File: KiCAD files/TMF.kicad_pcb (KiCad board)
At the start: 2 copper layers, 100 x 99.5 mm, 90 parts, among them J1 Conn_01x04_Pin, J2 Conn_01x04_Pin

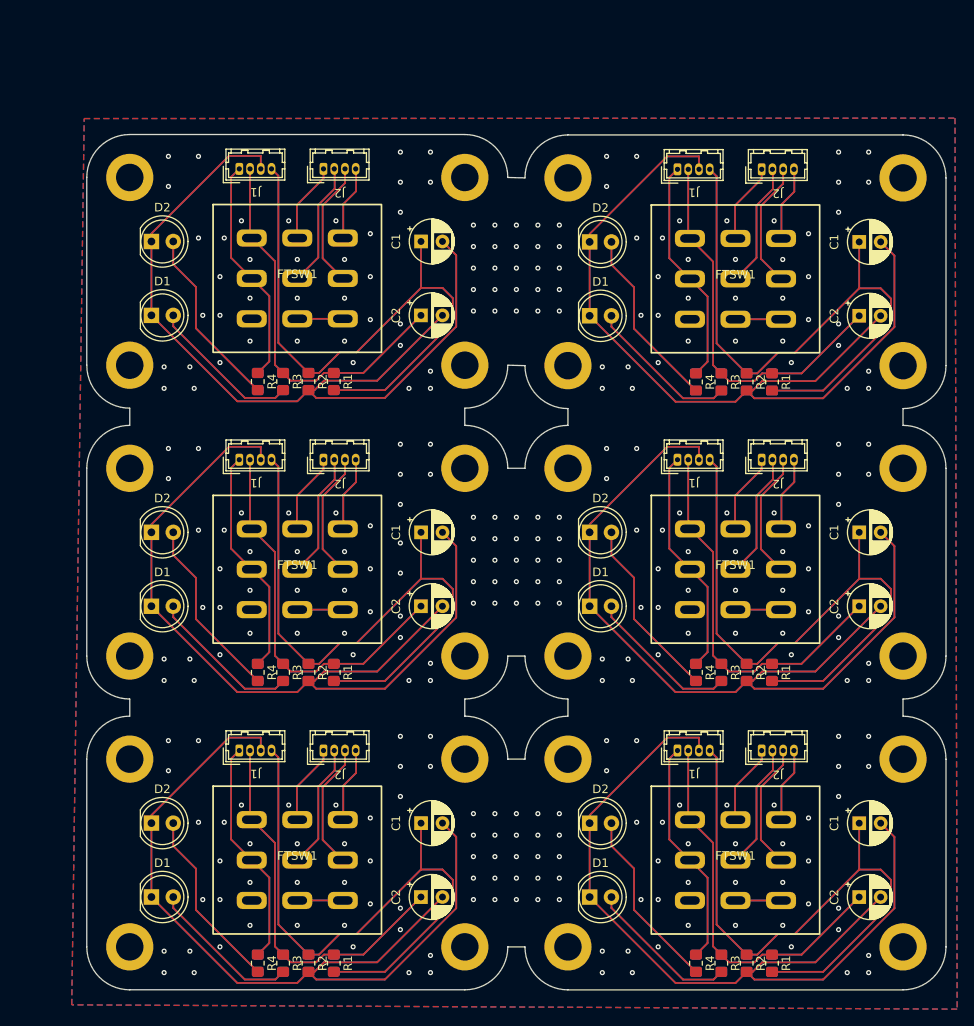
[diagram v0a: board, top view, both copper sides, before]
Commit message: Redone PCB
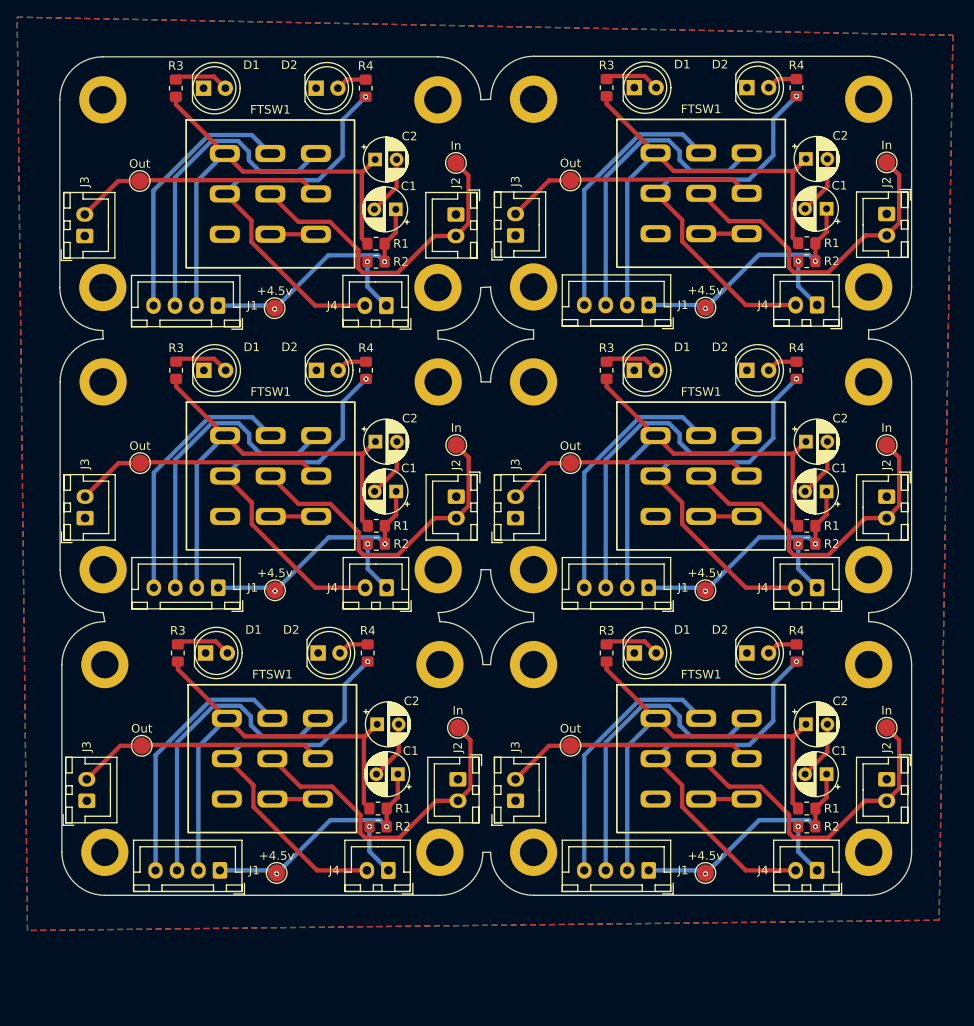
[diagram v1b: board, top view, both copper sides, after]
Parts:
- removed the ? at (167.0, 126.0)
- removed the ? at (167.0, 92.2)
- removed the ? at (116.0, 58.3)
- removed the ? at (167.0, 104.2)
- removed the ? at (116.0, 70.3)
- removed the ? at (116.0, 92.2)
- removed the ? at (116.0, 36.5)
- removed the ? at (167.0, 58.4)
- removed the ? at (167.0, 70.3)
- removed the ? at (167.0, 36.5)
- removed the C1 at (149.9, 43.9)
- removed the C1 at (149.9, 111.6)
- removed the C1 at (149.9, 77.8)
- removed the C1 at (200.9, 111.6)
- removed the C1 at (200.9, 44.0)
- removed the C1 at (200.9, 77.8)
- removed the C2 at (200.9, 86.4)
- removed the C2 at (149.9, 120.2)
- removed the C2 at (149.9, 52.5)
- removed the C2 at (149.9, 86.4)
- removed the C2 at (200.9, 120.2)
- removed the C2 at (200.9, 52.6)
- removed the D1 at (118.5, 86.4)
- removed the D1 at (118.5, 52.5)
- removed the D1 at (118.5, 120.2)
- removed the D1 at (169.5, 120.2)
- removed the D1 at (169.5, 86.4)
- removed the D1 at (169.5, 52.6)
- removed the D2 at (118.5, 77.8)
- removed the D2 at (118.5, 43.9)
- removed the D2 at (169.5, 111.6)
- removed the D2 at (118.5, 111.6)
- removed the D2 at (169.5, 77.8)
- removed the D2 at (169.5, 44.0)
- removed the FTSW1 at (135.5, 48.2)
- removed the FTSW1 at (186.5, 115.9)
- removed the FTSW1 at (135.5, 115.9)
- removed the FTSW1 at (186.5, 48.3)
- removed the FTSW1 at (186.5, 82.1)
- removed the FTSW1 at (135.5, 82.1)
- removed the J1 at (179.8, 35.5)
- removed the J1 at (128.8, 35.5)
- removed the J1 at (179.8, 103.2)
- removed the J1 at (128.8, 69.3)
- removed the J1 at (179.8, 69.3)
- removed the J1 at (128.8, 103.2)
- removed the J2 at (138.6, 35.5)
- removed the J2 at (189.6, 35.5)
- removed the J2 at (138.6, 69.3)
- removed the J2 at (138.6, 103.2)
- removed the J2 at (189.6, 103.2)
- removed the J2 at (189.6, 69.3)
- removed the R1 at (190.8, 60.3)
- removed the R1 at (190.8, 94.1)
- removed the R1 at (139.8, 127.9)
- removed the R1 at (139.8, 94.1)
- removed the R1 at (139.8, 60.2)
- removed the R1 at (190.8, 127.9)
- removed the R2 at (136.8, 94.1)
- removed the R2 at (187.8, 94.1)
- removed the R2 at (136.8, 60.2)
- removed the R2 at (187.8, 127.9)
- removed the R2 at (136.8, 127.9)
- removed the R2 at (187.8, 60.3)
- removed the R3 at (184.8, 94.1)
- removed the R3 at (133.8, 94.1)
- removed the R3 at (184.8, 127.9)
- removed the R3 at (133.8, 127.9)
- removed the R3 at (133.8, 60.2)
- removed the R3 at (184.8, 60.3)
- removed the R4 at (130.9, 60.2)
- removed the R4 at (181.9, 60.3)
- removed the R4 at (181.9, 127.9)
- removed the R4 at (130.9, 94.1)
- removed the R4 at (130.9, 127.9)
- removed the R4 at (181.9, 94.1)
- removed the REF** at (206.0, 70.3)
- removed the REF** at (155.0, 92.2)
- removed the REF** at (155.0, 70.3)
- removed the REF** at (206.0, 104.2)
- removed the REF** at (155.0, 58.3)
- removed the REF** at (206.0, 92.2)
- removed the REF** at (206.0, 58.4)
- removed the REF** at (206.0, 36.5)
- removed the REF** at (155.0, 36.5)
- removed the REF** at (206.0, 126.0)
- added +4.5v: TestPoint_Pad_D2.0mm, TestPoint:TestPoint_Pad_D2.0mm, F.Cu at (183.0, 117.4)
- added +4.5v: TestPoint_Pad_D2.0mm, TestPoint:TestPoint_Pad_D2.0mm, F.Cu at (132.9, 51.7)
- added +4.5v: TestPoint_Pad_D2.0mm, TestPoint:TestPoint_Pad_D2.0mm, F.Cu at (183.0, 51.6)
- added +4.5v: TestPoint_Pad_D2.0mm, TestPoint:TestPoint_Pad_D2.0mm, F.Cu at (183.0, 84.5)
- added +4.5v: TestPoint_Pad_D2.0mm, TestPoint:TestPoint_Pad_D2.0mm, F.Cu at (132.9, 84.5)
- added +4.5v: TestPoint_Pad_D2.0mm, TestPoint:TestPoint_Pad_D2.0mm, F.Cu at (133.1, 117.4)
- added ?: , , F.Cu at (112.9, 82.1)
- added ?: , , F.Cu at (112.9, 27.4)
- added ?: , , F.Cu at (112.9, 49.3)
- added ?: , , F.Cu at (163.0, 49.2)
- added ?: , , F.Cu at (163.0, 27.3)
- added ?: , , F.Cu at (163.0, 93.1)
- added ?: , , F.Cu at (163.0, 115.0)
- added ?: , , F.Cu at (112.9, 60.2)
- added ?: , , F.Cu at (163.0, 60.2)
- added ?: , , F.Cu at (163.0, 82.1)
- added C1: 10µF, Capacitor_THT:CP_Radial_D5.0mm_P2.50mm, F.Cu at (197.1, 40.1)
- added C1: 10µF, Capacitor_THT:CP_Radial_D5.0mm_P2.50mm, F.Cu at (147.0, 73.0)
- added C1: 10µF, Capacitor_THT:CP_Radial_D5.0mm_P2.50mm, F.Cu at (147.0, 40.2)
- added C1: 10µF, Capacitor_THT:CP_Radial_D5.0mm_P2.50mm, F.Cu at (147.2, 105.9)
- added C1: 10µF, Capacitor_THT:CP_Radial_D5.0mm_P2.50mm, F.Cu at (197.1, 105.9)
- added C1: 10µF, Capacitor_THT:CP_Radial_D5.0mm_P2.50mm, F.Cu at (197.1, 73.0)
- added C2: 100µF, Capacitor_THT:CP_Radial_D5.0mm_P2.50mm, F.Cu at (194.7, 34.3)
- added C2: 100µF, Capacitor_THT:CP_Radial_D5.0mm_P2.50mm, F.Cu at (194.7, 67.2)
- added C2: 100µF, Capacitor_THT:CP_Radial_D5.0mm_P2.50mm, F.Cu at (144.8, 100.1)
- added C2: 100µF, Capacitor_THT:CP_Radial_D5.0mm_P2.50mm, F.Cu at (194.7, 100.1)
- added C2: 100µF, Capacitor_THT:CP_Radial_D5.0mm_P2.50mm, F.Cu at (144.6, 34.4)
- added C2: 100µF, Capacitor_THT:CP_Radial_D5.0mm_P2.50mm, F.Cu at (144.6, 67.2)
- added D1: EFFECT, LED_THT:LED_D5.0mm_Clear, F.Cu at (124.6, 58.9)
- added D1: EFFECT, LED_THT:LED_D5.0mm_Clear, F.Cu at (174.7, 58.9)
- added D1: EFFECT, LED_THT:LED_D5.0mm_Clear, F.Cu at (124.8, 91.8)
- added D1: EFFECT, LED_THT:LED_D5.0mm_Clear, F.Cu at (174.7, 91.8)
- added D1: EFFECT, LED_THT:LED_D5.0mm_Clear, F.Cu at (124.6, 26.1)
- added D1: EFFECT, LED_THT:LED_D5.0mm_Clear, F.Cu at (174.7, 26.0)
- added D2: POW, LED_THT:LED_D5.0mm_Clear, F.Cu at (137.9, 91.8)
- added D2: POW, LED_THT:LED_D5.0mm_Clear, F.Cu at (137.7, 58.9)
- added D2: POW, LED_THT:LED_D5.0mm_Clear, F.Cu at (187.8, 58.9)
- added D2: POW, LED_THT:LED_D5.0mm_Clear, F.Cu at (187.8, 91.8)
- added D2: POW, LED_THT:LED_D5.0mm_Clear, F.Cu at (187.8, 26.0)
- added D2: POW, LED_THT:LED_D5.0mm_Clear, F.Cu at (137.7, 26.1)
- added FTSW1: ~, Footswitch:3PDT Footswitch, F.Cu at (132.6, 104.1)
- added FTSW1: ~, Footswitch:3PDT Footswitch, F.Cu at (182.5, 38.3)
- added FTSW1: ~, Footswitch:3PDT Footswitch, F.Cu at (182.5, 104.1)
- added FTSW1: ~, Footswitch:3PDT Footswitch, F.Cu at (132.4, 38.4)
- added FTSW1: ~, Footswitch:3PDT Footswitch, F.Cu at (182.5, 71.2)
- added FTSW1: ~, Footswitch:3PDT Footswitch, F.Cu at (132.4, 71.2)
- added In: TestPoint_Pad_D2.0mm, TestPoint:TestPoint_Pad_D2.0mm, F.Cu at (204.1, 34.7)
- added In: TestPoint_Pad_D2.0mm, TestPoint:TestPoint_Pad_D2.0mm, F.Cu at (154.0, 67.6)
- added In: TestPoint_Pad_D2.0mm, TestPoint:TestPoint_Pad_D2.0mm, F.Cu at (154.2, 100.5)
- added In: TestPoint_Pad_D2.0mm, TestPoint:TestPoint_Pad_D2.0mm, F.Cu at (204.1, 100.5)
- added In: TestPoint_Pad_D2.0mm, TestPoint:TestPoint_Pad_D2.0mm, F.Cu at (204.1, 67.6)
- added In: TestPoint_Pad_D2.0mm, TestPoint:TestPoint_Pad_D2.0mm, F.Cu at (154.0, 34.8)
- added J1: DST-2, Connector_JST:JST_XH_B4B-XH-A_1x04_P2.50mm_Vertical, F.Cu at (126.3, 51.4)
- added J1: DST-2, Connector_JST:JST_XH_B4B-XH-A_1x04_P2.50mm_Vertical, F.Cu at (176.4, 117.1)
- added J1: DST-2, Connector_JST:JST_XH_B4B-XH-A_1x04_P2.50mm_Vertical, F.Cu at (126.5, 117.1)
- added J1: DST-2, Connector_JST:JST_XH_B4B-XH-A_1x04_P2.50mm_Vertical, F.Cu at (176.4, 51.3)
- added J1: DST-2, Connector_JST:JST_XH_B4B-XH-A_1x04_P2.50mm_Vertical, F.Cu at (126.3, 84.2)
- added J1: DST-2, Connector_JST:JST_XH_B4B-XH-A_1x04_P2.50mm_Vertical, F.Cu at (176.4, 84.2)
- added J2: TMC-1, Connector_JST:JST_XH_B2B-XH-A_1x02_P2.50mm_Vertical, F.Cu at (154.2, 106.5)
- added J2: TMC-1, Connector_JST:JST_XH_B2B-XH-A_1x02_P2.50mm_Vertical, F.Cu at (204.1, 106.5)
- added J2: TMC-1, Connector_JST:JST_XH_B2B-XH-A_1x02_P2.50mm_Vertical, F.Cu at (204.1, 40.7)
- added J2: TMC-1, Connector_JST:JST_XH_B2B-XH-A_1x02_P2.50mm_Vertical, F.Cu at (154.0, 73.6)
- added J2: TMC-1, Connector_JST:JST_XH_B2B-XH-A_1x02_P2.50mm_Vertical, F.Cu at (204.1, 73.6)
- added J2: TMC-1, Connector_JST:JST_XH_B2B-XH-A_1x02_P2.50mm_Vertical, F.Cu at (154.0, 40.8)
- added J3: TMC-1, Connector_JST:JST_XH_B2B-XH-A_1x02_P2.50mm_Vertical, F.Cu at (160.9, 43.2)
- added J3: TMC-1, Connector_JST:JST_XH_B2B-XH-A_1x02_P2.50mm_Vertical, F.Cu at (160.9, 76.1)
- added J3: TMC-1, Connector_JST:JST_XH_B2B-XH-A_1x02_P2.50mm_Vertical, F.Cu at (160.9, 109.0)
- added J3: TMC-1, Connector_JST:JST_XH_B2B-XH-A_1x02_P2.50mm_Vertical, F.Cu at (110.8, 43.3)
- added J3: TMC-1, Connector_JST:JST_XH_B2B-XH-A_1x02_P2.50mm_Vertical, F.Cu at (111.0, 109.0)
- added J3: TMC-1, Connector_JST:JST_XH_B2B-XH-A_1x02_P2.50mm_Vertical, F.Cu at (110.8, 76.1)
- added J4: DST-2, Connector_JST:JST_XH_B2B-XH-A_1x02_P2.50mm_Vertical, F.Cu at (145.9, 51.4)
- added J4: DST-2, Connector_JST:JST_XH_B2B-XH-A_1x02_P2.50mm_Vertical, F.Cu at (196.0, 84.2)
- added J4: DST-2, Connector_JST:JST_XH_B2B-XH-A_1x02_P2.50mm_Vertical, F.Cu at (196.0, 117.1)
- added J4: DST-2, Connector_JST:JST_XH_B2B-XH-A_1x02_P2.50mm_Vertical, F.Cu at (145.9, 84.2)
- added J4: DST-2, Connector_JST:JST_XH_B2B-XH-A_1x02_P2.50mm_Vertical, F.Cu at (196.0, 51.3)
- added J4: DST-2, Connector_JST:JST_XH_B2B-XH-A_1x02_P2.50mm_Vertical, F.Cu at (146.1, 117.1)
- added Out: TestPoint_Pad_D2.0mm, TestPoint:TestPoint_Pad_D2.0mm, F.Cu at (167.3, 36.8)
- added Out: TestPoint_Pad_D2.0mm, TestPoint:TestPoint_Pad_D2.0mm, F.Cu at (117.4, 102.6)
- added Out: TestPoint_Pad_D2.0mm, TestPoint:TestPoint_Pad_D2.0mm, F.Cu at (117.2, 36.9)
- added Out: TestPoint_Pad_D2.0mm, TestPoint:TestPoint_Pad_D2.0mm, F.Cu at (117.2, 69.7)
- added Out: TestPoint_Pad_D2.0mm, TestPoint:TestPoint_Pad_D2.0mm, F.Cu at (167.3, 69.7)
- added Out: TestPoint_Pad_D2.0mm, TestPoint:TestPoint_Pad_D2.0mm, F.Cu at (167.3, 102.6)
- added R1: 10kΩ, Resistor_SMD:R_0805_2012Metric_Pad1.20x1.40mm_HandSolder, F.Cu at (194.8, 77.0)
- added R1: 10kΩ, Resistor_SMD:R_0805_2012Metric_Pad1.20x1.40mm_HandSolder, F.Cu at (144.9, 109.9)
- added R1: 10kΩ, Resistor_SMD:R_0805_2012Metric_Pad1.20x1.40mm_HandSolder, F.Cu at (194.8, 109.9)
- added R1: 10kΩ, Resistor_SMD:R_0805_2012Metric_Pad1.20x1.40mm_HandSolder, F.Cu at (144.7, 44.2)
- added R1: 10kΩ, Resistor_SMD:R_0805_2012Metric_Pad1.20x1.40mm_HandSolder, F.Cu at (144.7, 77.0)
- added R1: 10kΩ, Resistor_SMD:R_0805_2012Metric_Pad1.20x1.40mm_HandSolder, F.Cu at (194.8, 44.1)
- added R2: 10kΩ, Resistor_SMD:R_0805_2012Metric_Pad1.20x1.40mm_HandSolder, F.Cu at (194.8, 46.2)
- added R2: 10kΩ, Resistor_SMD:R_0805_2012Metric_Pad1.20x1.40mm_HandSolder, F.Cu at (144.7, 46.3)
- added R2: 10kΩ, Resistor_SMD:R_0805_2012Metric_Pad1.20x1.40mm_HandSolder, F.Cu at (194.8, 112.0)
- added R2: 10kΩ, Resistor_SMD:R_0805_2012Metric_Pad1.20x1.40mm_HandSolder, F.Cu at (194.8, 79.1)
- added R2: 10kΩ, Resistor_SMD:R_0805_2012Metric_Pad1.20x1.40mm_HandSolder, F.Cu at (144.7, 79.1)
- added R2: 10kΩ, Resistor_SMD:R_0805_2012Metric_Pad1.20x1.40mm_HandSolder, F.Cu at (144.9, 112.0)
- added R3: 1kΩ, Resistor_SMD:R_0805_2012Metric_Pad1.20x1.40mm_HandSolder, F.Cu at (171.5, 26.0)
- added R3: 1kΩ, Resistor_SMD:R_0805_2012Metric_Pad1.20x1.40mm_HandSolder, F.Cu at (171.5, 58.9)
- added R3: 1kΩ, Resistor_SMD:R_0805_2012Metric_Pad1.20x1.40mm_HandSolder, F.Cu at (121.6, 91.8)
- added R3: 1kΩ, Resistor_SMD:R_0805_2012Metric_Pad1.20x1.40mm_HandSolder, F.Cu at (121.4, 58.9)
- added R3: 1kΩ, Resistor_SMD:R_0805_2012Metric_Pad1.20x1.40mm_HandSolder, F.Cu at (171.5, 91.8)
- added R3: 1kΩ, Resistor_SMD:R_0805_2012Metric_Pad1.20x1.40mm_HandSolder, F.Cu at (121.4, 26.1)
- added R4: 1kΩ, Resistor_SMD:R_0805_2012Metric_Pad1.20x1.40mm_HandSolder, F.Cu at (193.6, 58.9)
- added R4: 1kΩ, Resistor_SMD:R_0805_2012Metric_Pad1.20x1.40mm_HandSolder, F.Cu at (193.6, 91.8)
- added R4: 1kΩ, Resistor_SMD:R_0805_2012Metric_Pad1.20x1.40mm_HandSolder, F.Cu at (143.5, 26.1)
- added R4: 1kΩ, Resistor_SMD:R_0805_2012Metric_Pad1.20x1.40mm_HandSolder, F.Cu at (143.5, 58.9)
- added R4: 1kΩ, Resistor_SMD:R_0805_2012Metric_Pad1.20x1.40mm_HandSolder, F.Cu at (143.7, 91.8)
- added R4: 1kΩ, Resistor_SMD:R_0805_2012Metric_Pad1.20x1.40mm_HandSolder, F.Cu at (193.6, 26.0)
- added REF**: MountingHole_3.2mm_M3_ISO14580_Pad, MountingHole:MountingHole_3.2mm_M3_ISO14580_Pad, F.Cu at (202.0, 115.0)
- added REF**: MountingHole_3.2mm_M3_ISO14580_Pad, MountingHole:MountingHole_3.2mm_M3_ISO14580_Pad, F.Cu at (202.0, 27.4)
- added REF**: MountingHole_3.2mm_M3_ISO14580_Pad, MountingHole:MountingHole_3.2mm_M3_ISO14580_Pad, F.Cu at (151.9, 82.1)
- added REF**: MountingHole_3.2mm_M3_ISO14580_Pad, MountingHole:MountingHole_3.2mm_M3_ISO14580_Pad, F.Cu at (151.9, 49.3)
- added REF**: MountingHole_3.2mm_M3_ISO14580_Pad, MountingHole:MountingHole_3.2mm_M3_ISO14580_Pad, F.Cu at (202.0, 82.1)
- added REF**: MountingHole_3.2mm_M3_ISO14580_Pad, MountingHole:MountingHole_3.2mm_M3_ISO14580_Pad, F.Cu at (202.0, 93.2)
- added REF**: MountingHole_3.2mm_M3_ISO14580_Pad, MountingHole:MountingHole_3.2mm_M3_ISO14580_Pad, F.Cu at (151.9, 60.3)
- added REF**: MountingHole_3.2mm_M3_ISO14580_Pad, MountingHole:MountingHole_3.2mm_M3_ISO14580_Pad, F.Cu at (202.0, 49.2)
- added REF**: MountingHole_3.2mm_M3_ISO14580_Pad, MountingHole:MountingHole_3.2mm_M3_ISO14580_Pad, F.Cu at (151.9, 27.4)
- added REF**: MountingHole_3.2mm_M3_ISO14580_Pad, MountingHole:MountingHole_3.2mm_M3_ISO14580_Pad, F.Cu at (202.0, 60.3)
- moved ? 11.4 mm to (113.1, 93.1)
- moved ? 11.4 mm to (113.1, 115.0)
- moved REF** 11.4 mm to (152.1, 93.2)
- moved REF** 11.4 mm to (152.1, 115.0)
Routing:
- net GND: track 1209.0 -> 77.3 mm, vias 311 -> 6
- net +4,5v: track 867.0 -> 174.6 mm, vias 0 -> 12
- net Net-(D2-A): track 256.5 -> 21.9 mm
- net +9v: track 538.9 -> 346.1 mm
- net Net-(D1-A): track 214.6 -> 38.8 mm
- net effect_out: track 104.8 -> 215.9 mm
- net effect_in: track 112.3 -> 183.3 mm
- net in: track 174.7 -> 228.7 mm
- net +batt: track 318.6 -> 282.7 mm, vias 0 -> 6
- net clean: track 63.6 -> 31.8 mm
- net out: track 177.6 -> 174.5 mm
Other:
- board size 100 x 99.5 mm -> 99.1 x 97.7 mm
